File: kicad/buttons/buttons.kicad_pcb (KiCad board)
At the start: 2 copper layers, 70 x 20 mm, 1 part

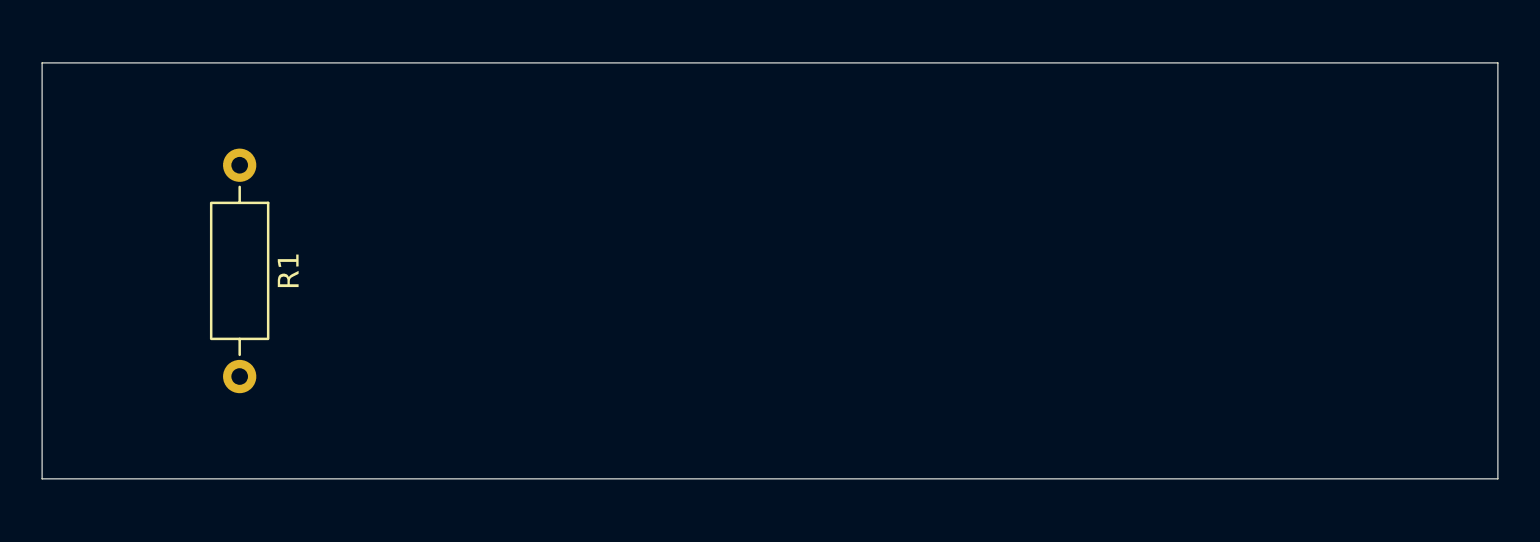
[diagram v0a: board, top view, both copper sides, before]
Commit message: finish buttons board
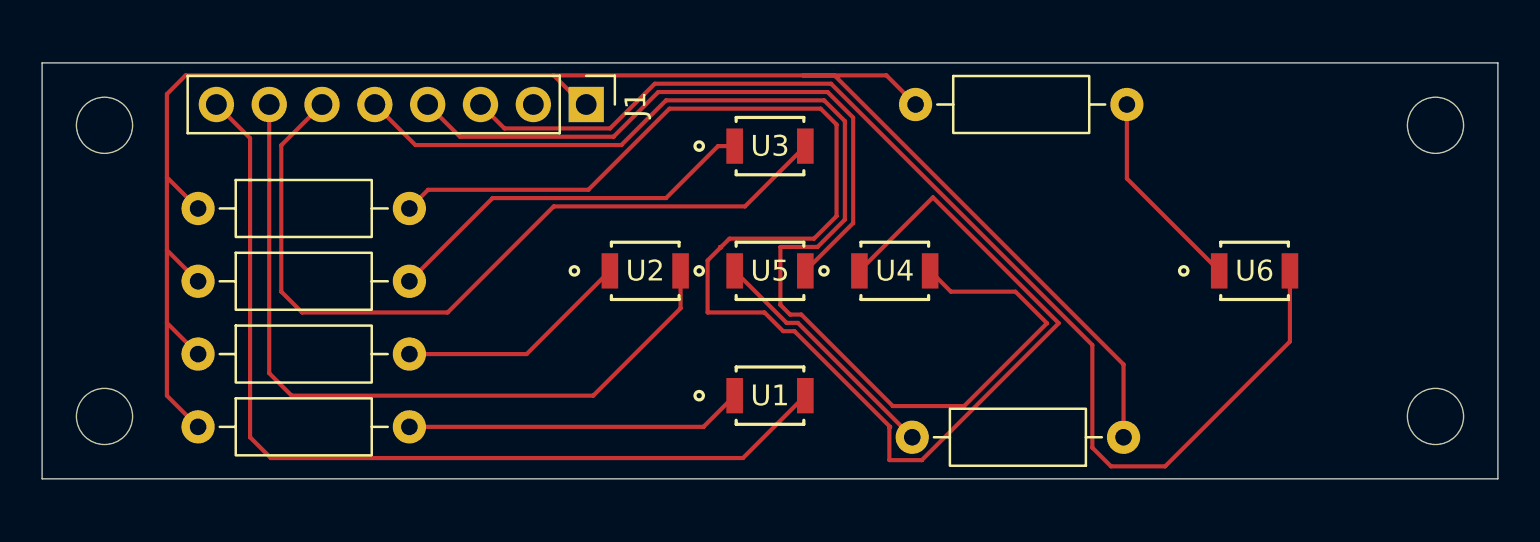
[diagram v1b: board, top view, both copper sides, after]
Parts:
- added J1: Conn_01x08_Pin, Connector_PinHeader_2.54mm:PinHeader_1x08_P2.54mm_Vertical, F.Cu at (101.2, 92.0)
- added MH2: MountingHole_2.7mm_M2.5, MountingHole:MountingHole_2.7mm_M2.5, F.Cu at (142.0, 93.0)
- added MH2: MountingHole_2.7mm_M2.5, MountingHole:MountingHole_2.7mm_M2.5, F.Cu at (78.0, 93.0)
- added MH2: MountingHole_2.7mm_M2.5, MountingHole:MountingHole_2.7mm_M2.5, F.Cu at (78.0, 107.0)
- added MH2: MountingHole_2.7mm_M2.5, MountingHole:MountingHole_2.7mm_M2.5, F.Cu at (142.0, 107.0)
- added R2: R, Resistor_THT:R_Axial_DIN0207_L6.3mm_D2.5mm_P10.16mm_Horizontal, F.Cu at (82.5, 104.0)
- added R3: R, Resistor_THT:R_Axial_DIN0207_L6.3mm_D2.5mm_P10.16mm_Horizontal, F.Cu at (82.5, 100.5)
- added R4: R, Resistor_THT:R_Axial_DIN0207_L6.3mm_D2.5mm_P10.16mm_Horizontal, F.Cu at (82.5, 97.0)
- added R5: R, Resistor_THT:R_Axial_DIN0207_L6.3mm_D2.5mm_P10.16mm_Horizontal, F.Cu at (127.0, 108.0)
- added R6: R, Resistor_THT:R_Axial_DIN0207_L6.3mm_D2.5mm_P10.16mm_Horizontal, F.Cu at (117.0, 92.0)
- added U1: B3U-1000P, Omron:B3U-1000P, F.Cu at (110.0, 106.0)
- added U2: B3U-1000P, Omron:B3U-1000P, F.Cu at (104.0, 100.0)
- added U3: B3U-1000P, Omron:B3U-1000P, F.Cu at (110.0, 94.0)
- added U4: B3U-1000P, Omron:B3U-1000P, F.Cu at (116.0, 100.0)
- added U5: B3U-1000P, Omron:B3U-1000P, F.Cu at (110.0, 100.0)
- added U6: B3U-1000P, Omron:B3U-1000P, F.Cu at (133.3, 100.0)
- moved R1 12.7 mm to (82.5, 107.5), turned to 0 degrees
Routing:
- net Net-(J1-Pin_1): track 0.00 -> 86.7 mm
- net Net-(R4-Pad2): track 0.00 -> 74.0 mm
- net /Btn4: track 0.00 -> 59.0 mm
- net /Btn6: track 0.00 -> 56.7 mm
- net /Btn1: track 0.00 -> 45.0 mm
- net /Btn3: track 0.00 -> 38.7 mm
- net /Btn2: track 0.00 -> 36.7 mm
- net /Btn5: track 0.00 -> 30.8 mm
- net Net-(R3-Pad2): track 0.00 -> 18.3 mm
- net Net-(R1-Pad2): track 0.00 -> 16.3 mm
- net Net-(R5-Pad2): track 0.00 -> 11.9 mm
- net Net-(R2-Pad2): track 0.00 -> 11.3 mm
- net Net-(R6-Pad2): track 0.00 -> 9.84 mm

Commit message: improve buttons board
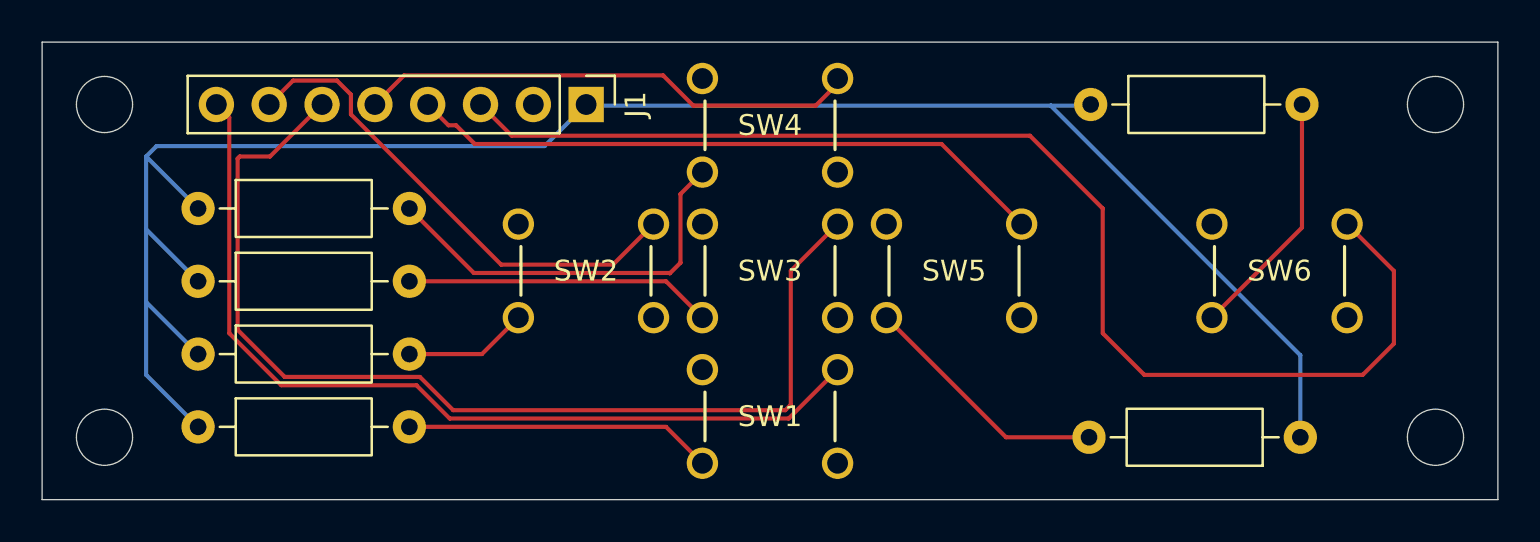
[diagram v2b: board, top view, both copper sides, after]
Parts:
- removed U1, U2, U3, U4, U5, U6: B3U-1000P, Omron:B3U-1000P
- added SW1: B3W-1000, Omron:SW_B3W-1000_OMR, F.Cu at (106.7, 104.8)
- added SW2: B3W-1000, Omron:SW_B3W-1000_OMR, F.Cu at (97.9, 97.8)
- added SW3: B3W-1000, Omron:SW_B3W-1000_OMR, F.Cu at (106.8, 97.8)
- added SW4: B3W-1000, Omron:SW_B3W-1000_OMR, F.Cu at (106.8, 90.8)
- added SW5: B3W-1000, Omron:SW_B3W-1000_OMR, F.Cu at (115.6, 97.8)
- added SW6: B3W-1000, Omron:SW_B3W-1000_OMR, F.Cu at (131.2, 97.8)
- moved R5 8.50 mm to (135.5, 108.0)
- moved R6 8.42 mm to (125.4, 92.0)
- moved MH2 1.00 mm to (142.0, 92.0)
- moved MH2 1.00 mm to (78.0, 92.0)
- moved MH2 1.00 mm to (78.0, 108.0)
- moved MH2 1.00 mm to (142.0, 108.0)
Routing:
- net Net-(R4-Pad2): track 74.0 -> 19.3 mm
- net /Btn4: track 59.0 -> 23.9 mm
- net /Btn2: track 36.7 -> 24.0 mm
- net /Btn3: track 38.7 -> 51.3 mm
- net Net-(R2-Pad2): track 11.3 -> 5.96 mm
- net Net-(J1-Pin_1): track 86.7 -> 92.1 mm
- net Net-(R3-Pad2): track 18.3 -> 14.8 mm
- net /Btn6: track 56.7 -> 60.1 mm
- net Net-(R6-Pad2): track 9.84 -> 12.0 mm
- net /Btn1: track 45.0 -> 43.2 mm
- net Net-(R1-Pad2): track 16.3 -> 14.8 mm
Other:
- board size 70 x 20 mm -> 70 x 22 mm
